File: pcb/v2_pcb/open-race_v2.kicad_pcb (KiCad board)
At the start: 8 copper layers, 90.5 x 49.5 mm, 337 parts, among them IC1 AP33772SDKZ-13-FA02, J1 Conn_ARM_SWD_TagConnect_TC203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, J2 USB4105-GF-A, J20 2S_PACK_BALANCE, J3 DM3CS-SF, J800 M50-3530642 (VTREF sense only), J900 U.FL-R-SMT-1(10), Q1 CSD18540Q5B, Q2 CSD18540Q5B, Q3 CSD18540Q5B, Q4 CSD18540Q5B, Q5 CSD18540Q5B, SW1101 KMR223NG ULC LFG, SW1102 KMR223NG ULC LFG, SW1103 KMR223NG ULC LFG, SW300 KMR223NG ULC LFG, SW301 KMR223NG ULC LFG, SW800 KMR223NG ULC LFG, SW801 KMR223NG ULC LFG, U1 STM32N657X0H3Q, U10 TPSM863253RDXR, U1000 SCH16T-K01-1, U11 TPS22997RYZR, U1100 SN74AHCT1G125DCKR, U1101 SN74AHCT1G125DCKR, U20 TPS630701RNMR (5V fixed), U21 TPS22918DBVR, U22 TPS22918DBVR, U23 TPS22918DBVR, U24 TXS0104EPW, U25 TPS3808G01DBVR, U26 TLV75533PDBVR, U3 APS512XXN-OB9-BG, U4 TPD8S300ARUKR, U5 IS25WP512M-RHLE, U6 BQ25798RQMR, U7 MAX17320G22+, U8 RPL-3.0-R, U800 ESP32-C6-MINI-1, U900 UM980, Y1 NX2016SA-24MHZ-EXS00A-CS10820, Y2 NX2012SA-32.768KHZ-EXS00A-MU0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

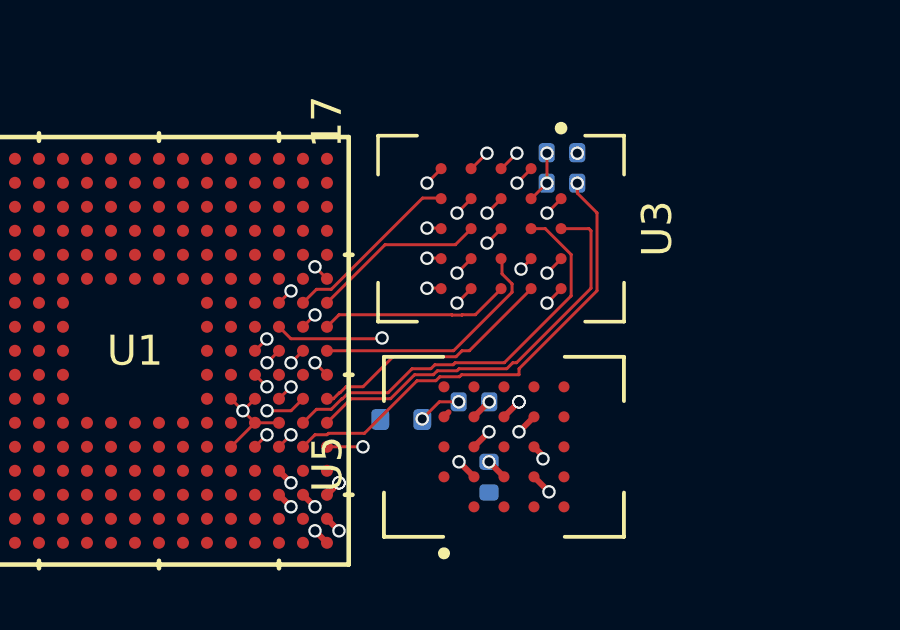
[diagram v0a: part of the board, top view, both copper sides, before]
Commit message: lengthmatch
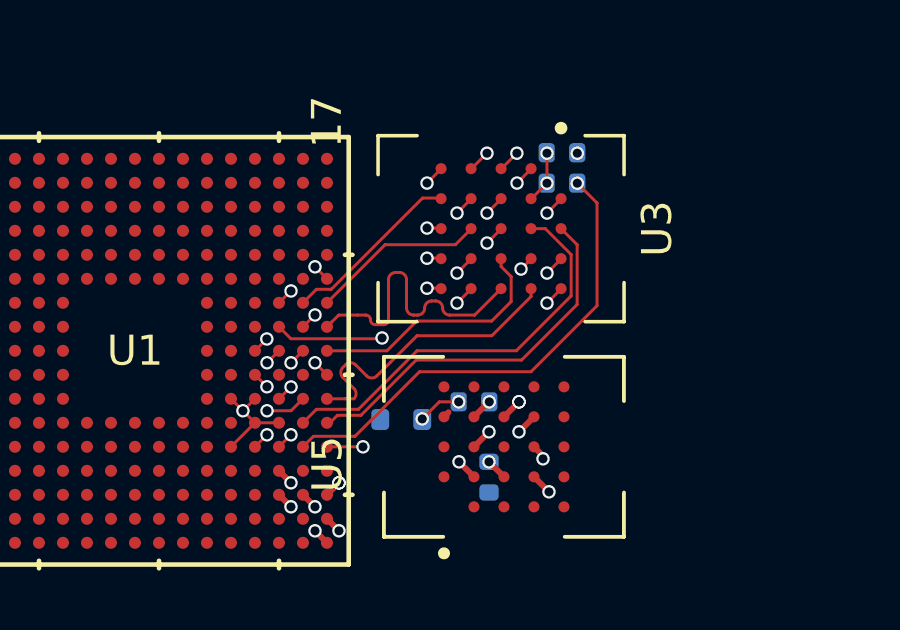
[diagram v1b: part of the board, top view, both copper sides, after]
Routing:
- net /STM32 MCU IO/PSRAM_IO15: track 6.38 -> 9.75 mm
- net /STM32 MCU IO/PSRAM_IO14: track 8.36 -> 10.0 mm
- net /STM32 MCU IO/PSRAM_NCS: track 13.6 -> 12.7 mm
